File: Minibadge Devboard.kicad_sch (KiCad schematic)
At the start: 41 parts, among them J1 External power, J2 External switch, SW1 Power, SW3 SPEED, SW4 NTC

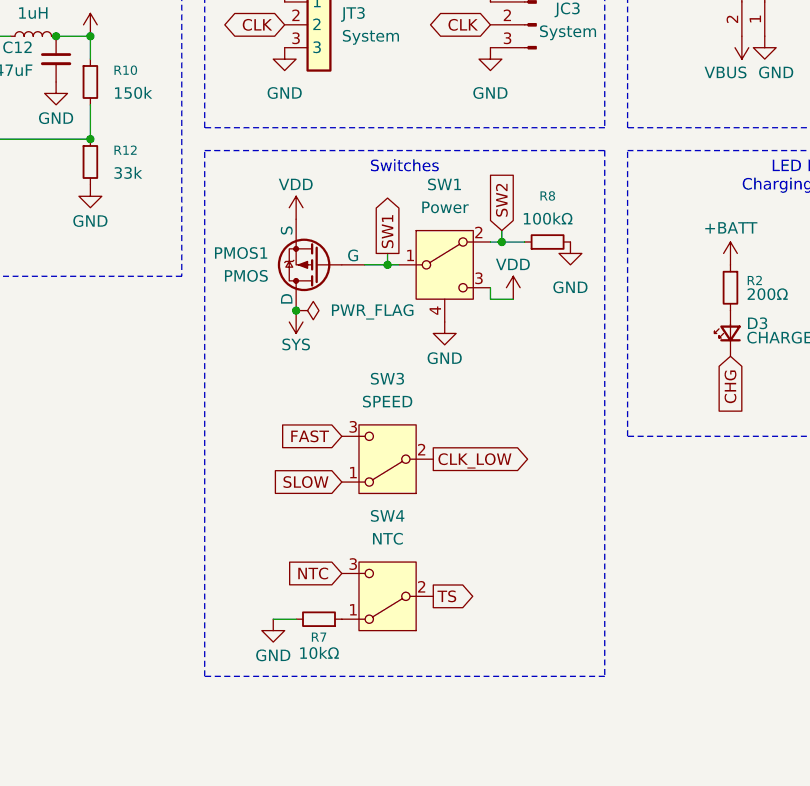
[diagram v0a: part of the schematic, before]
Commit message: update PDF
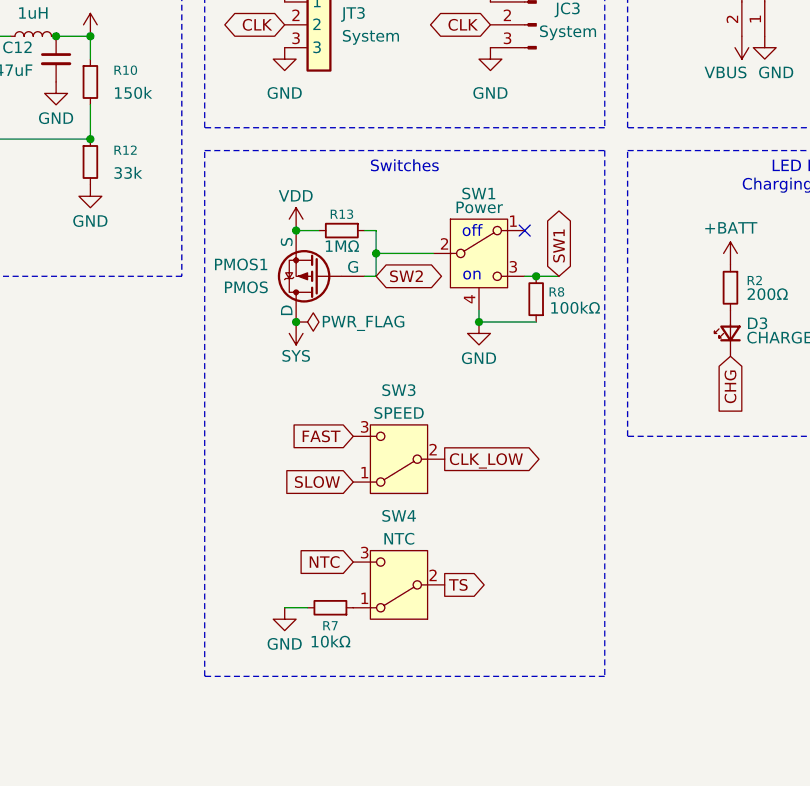
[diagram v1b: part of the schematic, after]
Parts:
- added R13: 1MΩ, Resistor_SMD:R_0603_1608Metric, symbol Device:R_Small
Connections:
- net GND: now also R8.1; no longer R8.2
- net SW1: now also R8.2, SW1.3 (C); no longer PMOS1.1 (G), SW1.1 (B)
- net SW2: now also PMOS1.1 (G), R13.1; no longer R8.1
- net VDD: now also R13.2; no longer SW1.3 (C)
- no-connect marks 10 -> 11
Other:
- note added: "off"
- note added: "on"
- moved on the sheet: PMOS1, R7, R8, SW1, SW3, SW4
